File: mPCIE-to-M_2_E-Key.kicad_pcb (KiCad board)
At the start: 2 copper layers, 10 parts, among them J2 Bus_M.2_Socket_E, Q1 BSS138K, Q2 BSS138K, U1 TL1963A

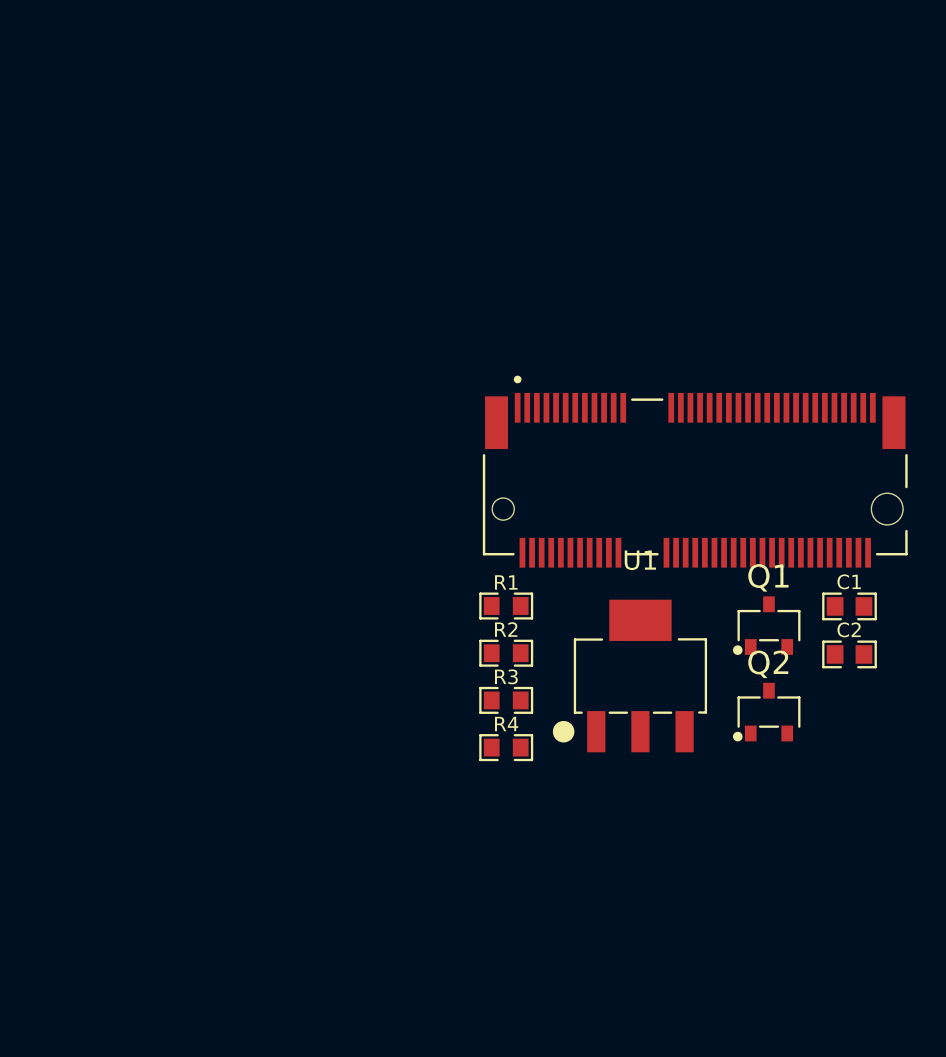
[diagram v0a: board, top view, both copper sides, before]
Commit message: updated files
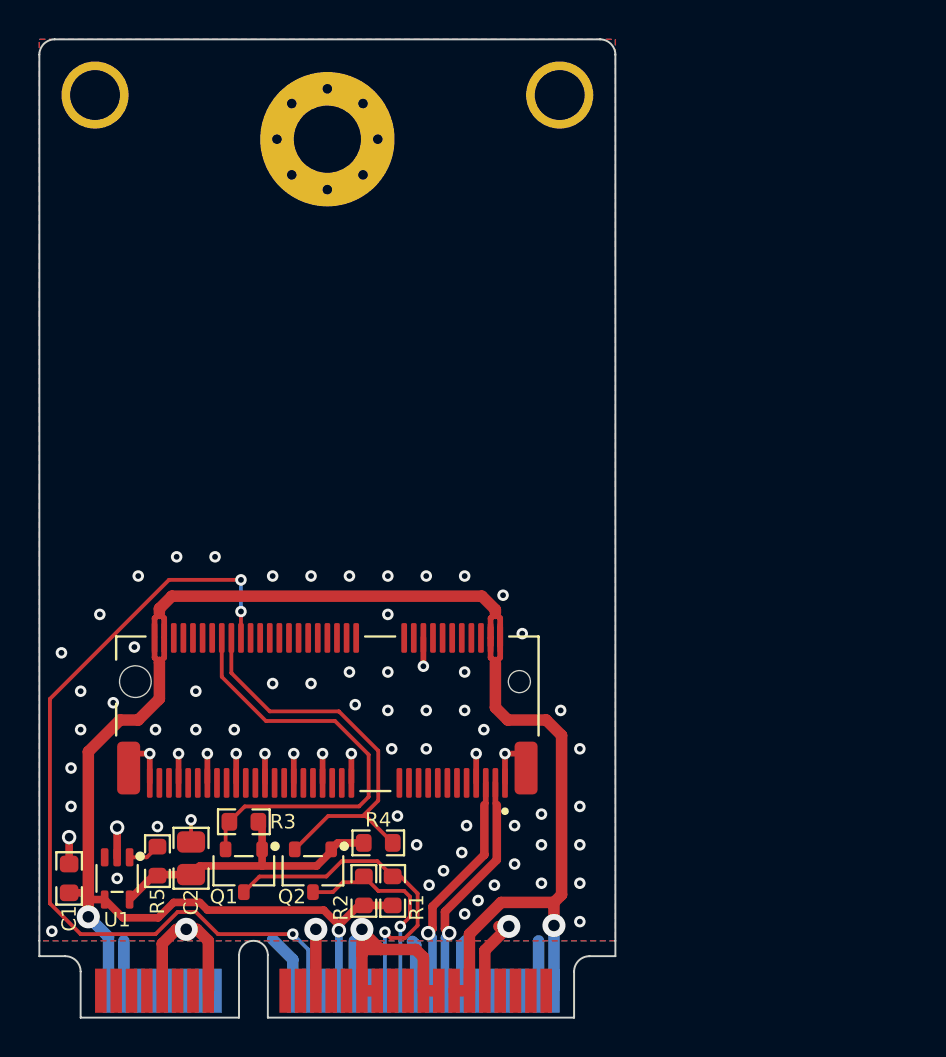
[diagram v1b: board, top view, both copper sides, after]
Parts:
- added H1: M2.5, lib_fp:M2.5_MH, F.Cu at (145.9, 82.0)
- added H2: M2.5, lib_fp:M2.5_MH, F.Cu at (121.8, 82.0)
- added H3: M3.5, lib_fp:MountingHole_3.5mm_Pad_Via, F.Cu at (133.8, 84.2)
- added J1: Bus_PCI_Express_Mini, lib_fp:BUS_mPCIe, F.Cu at (130.0, 130.0)
- added R5: 100K, lib_fp:CRCW0603, F.Cu at (125.0, 121.8)
- C1: value 10uF -> 100nF; footprint lib_fp:CAPC160X80X88L35N -> lib_fp:MLCC0603
- C2: value 10uF -> 470nF; footprint lib_fp:CAPC160X80X88L35N -> lib_fp:MLCC0805
- R1, R2, R3, R4: footprint lib_fp:RESC160X80X55L30N -> lib_fp:CRCW0603
- U1: value TL1963A -> TPS79718; footprint lib_fp:SOT223-4 -> lib_fp:SOT323-65P210X110-5
- moved C1 43.0 mm to (120.4, 122.8), turned to 90 degrees
- moved C2 35.9 mm to (126.8, 121.7), turned to 90 degrees
- moved Q1 30.2 mm to (129.5, 122.3), turned to 180 degrees
- moved U1 29.2 mm to (122.9, 122.8), turned to 180 degrees
- moved Q2 25.1 mm to (133.1, 122.3), turned to 180 degrees
- moved J2 21.2 mm to (133.8, 112.5), turned to 180 degrees
- moved R1 16.0 mm to (137.2, 123.4), turned to 90 degrees
- moved R3 15.1 mm to (129.5, 119.8), turned to 180 degrees
- moved R2 14.4 mm to (135.8, 123.4), turned to 90 degrees
- moved R4 8.31 mm to (136.5, 120.9)
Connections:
- net Net-(Q1-Pad3) renamed /SCL_3V3
- net Net-(Q2-Pad3) renamed /SDA_3V3
- J2 pad S1: Net-(J2-PadS1) -> GND
- J2 pad S2: Net-(J2-PadS1) -> GND
- Q1 pad 2: Net-(Q1-Pad2) -> /SCL_1V8
- Q2 pad 2: Net-(Q2-Pad2) -> /SDA_1V8
- R3 pad 2: Net-(Q1-Pad2) -> /SCL_1V8
- R4 pad 2: Net-(Q2-Pad2) -> /SDA_1V8
- U1 pad 1: +3V3 -> Net-(U1-PG)
- U1 pad 3: +1V8 -> unconnected-(U1-NC-Pad3)
- U1 pad 4: GND -> +3V3
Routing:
- net +3V3: track 0.00 -> 101.5 mm, vias 0 -> 3
- net GND: track 0.00 -> 66.2 mm, vias 0 -> 77
- net /W_DISABLE: track 0.00 -> 43.7 mm, vias 0 -> 3
- net /SCL_1V8: track 0.00 -> 22.8 mm
- net /SDA_1V8: track 0.00 -> 21.3 mm
- net /SCL_3V3: track 0.00 -> 17.3 mm, vias 0 -> 1
- net +1V8: track 0.00 -> 16.0 mm
- net /D_P: track 0.00 -> 12.2 mm, vias 0 -> 1
- net /D_N: track 0.00 -> 12.1 mm, vias 0 -> 1
- net /SDA_3V3: track 0.00 -> 11.2 mm, vias 0 -> 1
- net Net-(U1-PG): track 0.00 -> 1.68 mm
- added copper zone on B.Cu, net GND
- added copper zone on F.Cu, net GND
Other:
- board outline added: 30 x 47 mm
